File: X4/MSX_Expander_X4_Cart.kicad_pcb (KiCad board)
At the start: 2 copper layers, 103 x 66 mm, 17 parts, among them J1 MSX Edge Connector, J2 IDC50P - MSX BUS, U1 74LS273, U2 74LS540, U3 74LS352, U4 74LS139, U5 74LS11, U6 74LS133, U7 74LS32

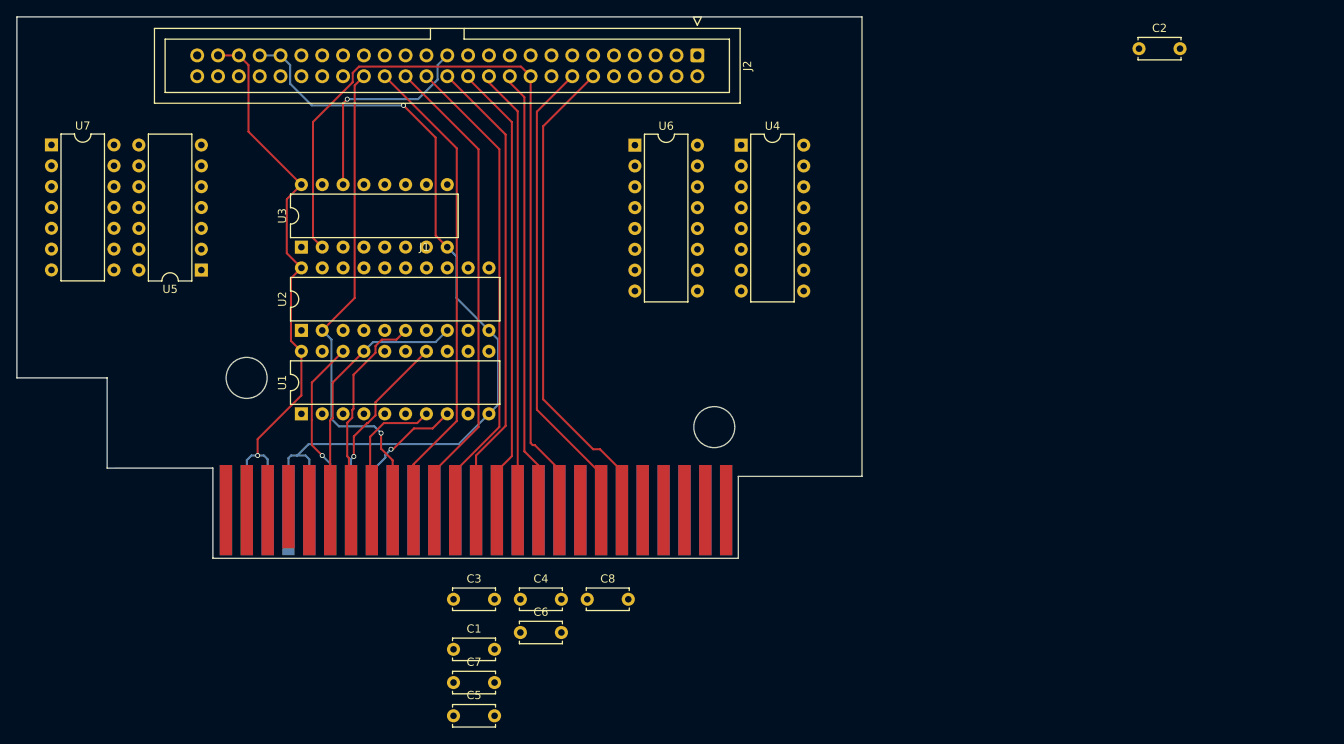
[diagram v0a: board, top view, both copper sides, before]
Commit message: started routing
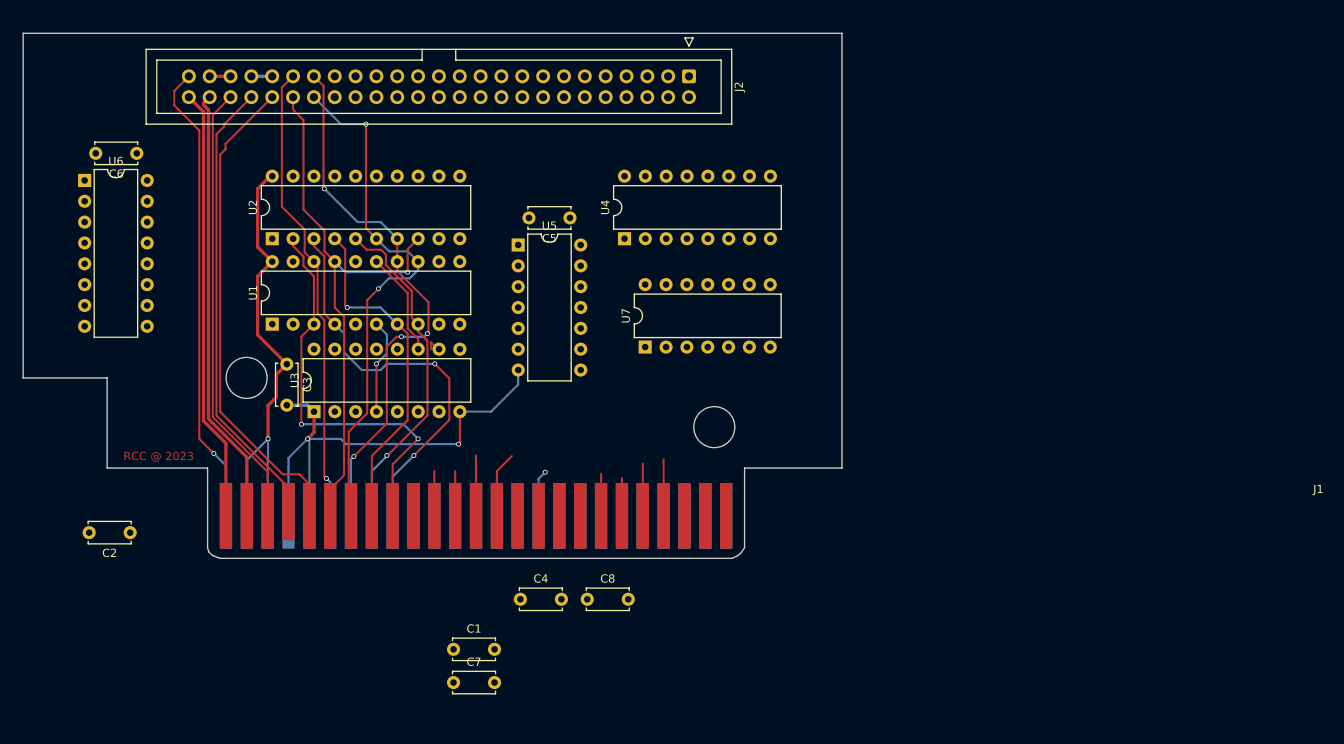
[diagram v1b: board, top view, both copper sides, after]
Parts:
- J1: footprint Roni Footprints:MSX_CART_SW -> Roni Footprints:MSX_CART_SW_Official
- moved C2 136.4 mm to (108.4, 105.9), turned to 180 degrees
- moved U7 76.4 mm to (171.2, 83.3), turned to 90 degrees
- moved C6 74.8 mm to (109.2, 59.7), turned to 180 degrees
- moved U6 67.2 mm to (102.9, 63.0)
- moved C5 62.3 mm to (162.0, 67.6), turned to 180 degrees
- moved U5 38.7 mm to (155.7, 70.9), turned to 0 degrees
- moved C3 35.1 mm to (127.5, 85.4), turned to -90 degrees
- moved U3 20.1 mm to (130.8, 91.2)
- moved U4 18.2 mm to (168.7, 70.1), turned to 90 degrees
- moved U2 11.7 mm to (125.7, 70.1)
- moved U1 11.5 mm to (125.7, 80.5)
- moved J2 2.74 mm to (176.5, 50.3)
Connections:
- U6 pad 16: (no net) -> +5V
- U6 pad 8: (no net) -> GND
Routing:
- net A15: track 100.7 -> 0.29 mm
- net CLOCK: track 0.00 -> 59.3 mm
- net A4: track 58.7 -> 0.00 mm
- net SOUNDIN: track 0.00 -> 56.9 mm, vias 0 -> 1
- net /MERQ: track 59.9 -> 3.91 mm
- net SW1: track 0.00 -> 55.9 mm
- net SW2: track 0.00 -> 54.7 mm
- net A6: track 54.3 -> 0.00 mm
- net A2: track 58.8 -> 4.75 mm
- net A0: track 58.8 -> 4.75 mm
- net A10: track 54.3 -> 0.65 mm
- net +12V: track 0.00 -> 53.5 mm
- net /RD: track 57.9 -> 4.42 mm
- net -12V: track 0.00 -> 52.9 mm
- net A13: track 57.3 -> 6.65 mm
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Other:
- board size 103 x 66 mm -> 99.8 x 64 mm
